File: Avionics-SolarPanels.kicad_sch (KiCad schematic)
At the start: 6 parts

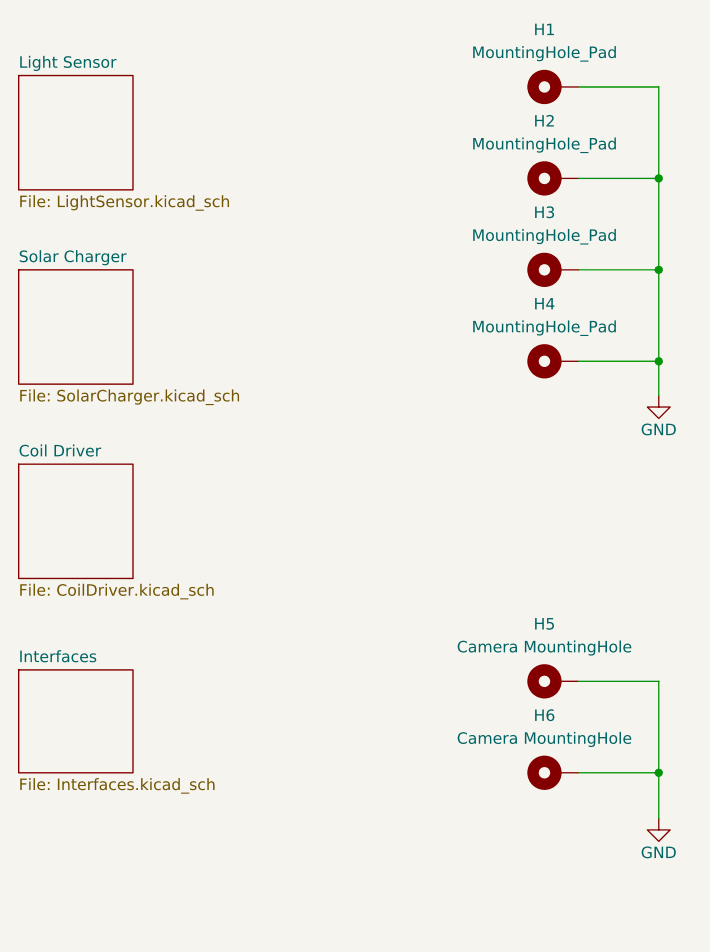
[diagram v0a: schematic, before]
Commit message: v3.1 Updates
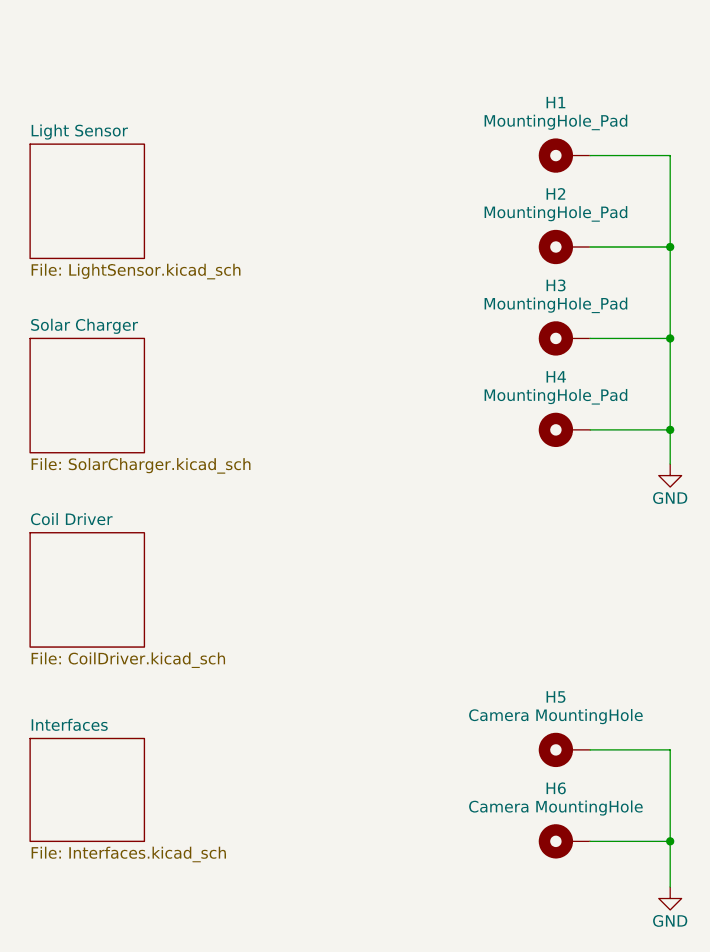
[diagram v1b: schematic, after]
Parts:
- H1, H4: footprint MountingHole:MountingHole_3.2mm_M3_DIN965_Pad_TopBottom -> Argus-Miscellaneous:MountingHole_3.2mm_5.2mm_Slot_TopBottom
- H5, H6: footprint MountingHole:MountingHole_3mm_Pad_TopBottom -> MountingHole:MountingHole_2.2mm_M2_DIN965_Pad_TopOnly
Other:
- company: (none) -> Carnegie Mellon University
- title: (none) -> Argus XY Solar Panel
- moved on the sheet: H1, H2, H3, H4, H5, H6
